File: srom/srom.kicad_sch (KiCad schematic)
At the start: 20 parts, among them J1 Conn_01x03_Female, Q1 PMBT2222A, U1 4075, U101 74LS245, U4 74LS245, U5 Pico-1 ROM

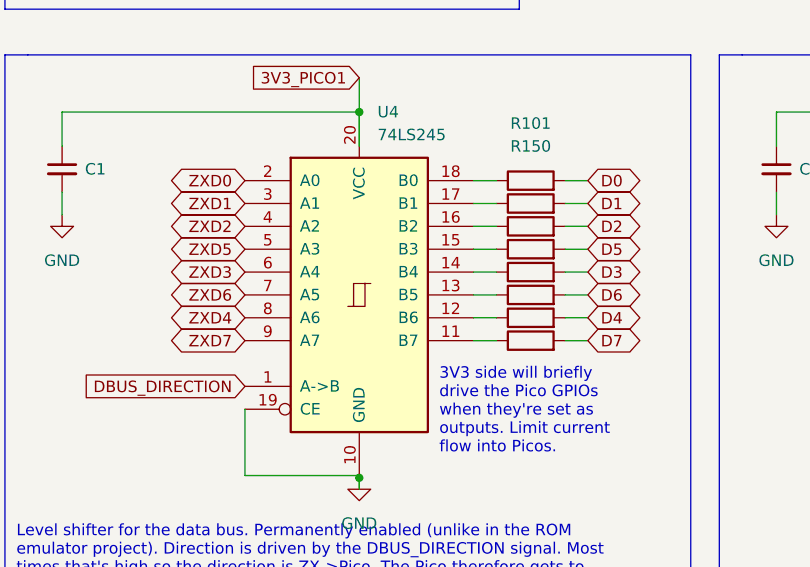
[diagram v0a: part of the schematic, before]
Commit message: first draft of layout of board 2
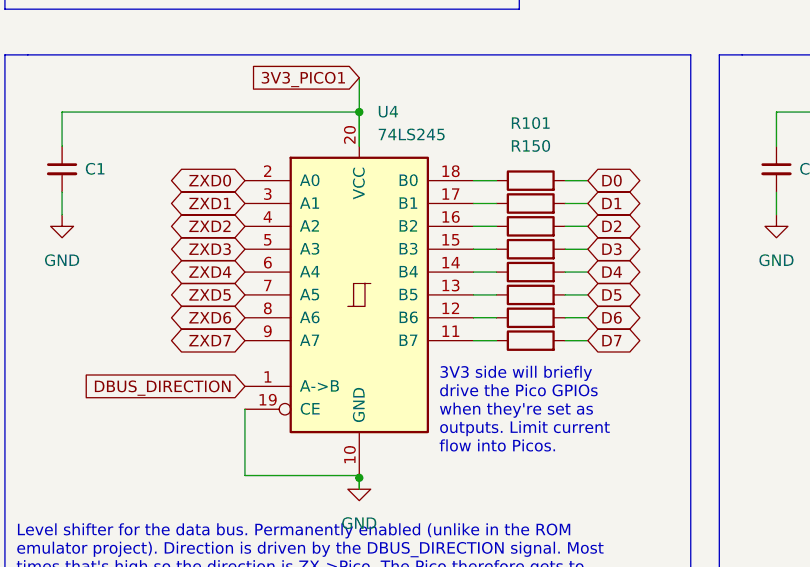
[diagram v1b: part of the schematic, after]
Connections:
- net D3: now also R104.2; no longer R105.2
- net D4: now also R105.2; no longer R107.2
- net D5: now also R106.2; no longer R104.2
- net D6: now also R107.2; no longer R106.2
- net ZXD3: now also U4.5 (A3); no longer U4.6 (A4)
- net ZXD4: now also U4.6 (A4); no longer U4.8 (A6)
- net ZXD5: now also U4.7 (A5); no longer U4.5 (A3)
- net ZXD6: now also U4.8 (A6); no longer U4.7 (A5)
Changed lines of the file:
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@@
     )
   )
-  (global_label "D4" (shape bidirectional) (at 78.74 138.43 0) (fields_autoplaced)
+  (global_label "D6" (shape bidirectional) (at 78.74 138.43 0) (fields_autoplaced)
     (effects (font (size 1.27 1.27)) (justify left))
     (property "Intersheet References" "${INTERSHEET_REFS}" (id 0) (at 83.6326 138.3506 0)
@@
     )
   )
-  (global_label "ZXD6" (shape bidirectional) (at 40.64 135.89 180) (fields_autoplaced)
+  (global_label "ZXD5" (shape bidirectional) (at 40.64 135.89 180) (fields_autoplaced)
     (effects (font (size 1.27 1.27)) (justify right))
     (property "Intersheet References" "${INTERSHEET_REFS}" (id 0) (at 33.3283 135.8106 0)
@@
     )
   )
-  (global_label "ZXD4" (shape bidirectional) (at 40.64 138.43 180) (fields_autoplaced)
+  (global_label "ZXD6" (shape bidirectional) (at 40.64 138.43 180) (fields_autoplaced)
     (effects (font (size 1.27 1.27)) (justify right))
     (property "Intersheet References" "${INTERSHEET_REFS}" (id 0) (at 33.3283 138.3506 0)
@@
     )
   )
-  (global_label "D3" (shape bidirectional) (at 78.74 133.35 0) (fields_autoplaced)
+  (global_label "D4" (shape bidirectional) (at 78.74 133.35 0) (fields_autoplaced)
     (effects (font (size 1.27 1.27)) (justify left))
     (property "Intersheet References" "${INTERSHEET_REFS}" (id 0) (at 83.6326 133.2706 0)
@@
     )
   )
-  (global_label "ZXD5" (shape bidirectional) (at 40.64 130.81 180) (fields_autoplaced)
+  (global_label "ZXD3" (shape bidirectional) (at 40.64 130.81 180) (fields_autoplaced)
     (effects (font (size 1.27 1.27)) (justify right))
     (property "Intersheet References" "${INTERSHEET_REFS}" (id 0) (at 33.3283 130.7306 0)
@@
     )
   )
-  (global_label "D6" (shape bidirectional) (at 78.74 135.89 0) (fields_autoplaced)
+  (global_label "D5" (shape bidirectional) (at 78.74 135.89 0) (fields_autoplaced)
     (effects (font (size 1.27 1.27)) (justify left))
     (property "Intersheet References" "${INTERSHEET_REFS}" (id 0) (at 83.6326 135.8106 0)
@@
     )
   )
-  (global_label "D5" (shape bidirectional) (at 78.74 130.81 0) (fields_autoplaced)
+  (global_label "D3" (shape bidirectional) (at 78.74 130.81 0) (fields_autoplaced)
     (effects (font (size 1.27 1.27)) (justify left))
     (property "Intersheet References" "${INTERSHEET_REFS}" (id 0) (at 83.6326 130.7306 0)
@@
     )
   )
-  (global_label "ZXD3" (shape bidirectional) (at 40.64 133.35 180) (fields_autoplaced)
+  (global_label "ZXD4" (shape bidirectional) (at 40.64 133.35 180) (fields_autoplaced)
     (effects (font (size 1.27 1.27)) (justify right))
     (property "Intersheet References" "${INTERSHEET_REFS}" (id 0) (at 33.3283 133.2706 0)
@@
       (reference "#PWR0201") (unit 1) (value "GND") (footprint "")
     )
+    (path "/95a6eb69-d4c1-4a7e-a8e8-144430faf0e2/49643f1b-a3e7-406d-9651-75cb8bc3c20f"
+      (reference "#PWR0202") (unit 1) (value "GND") (footprint "")
+    )
     (path "/95a6eb69-d4c1-4a7e-a8e8-144430faf0e2/b4561307-559f-491e-95d1-1c57e89e9bd0"
       (reference "#PWR0203") (unit 1) (value "GND") (footprint "")
@@
       (reference "C101") (unit 1) (value "C_Small") (footprint "Capacitor_SMD:C_1206_3216Metric")
     )
+    (path "/95a6eb69-d4c1-4a7e-a8e8-144430faf0e2/bc372065-041b-4223-9621-9581521839ff"
+      (reference "C201") (unit 1) (value "C_Small") (footprint "Capacitor_SMD:C_1206_3216Metric")
+    )
     (path "/986f0686-4dd2-4d11-a20b-857347ffd112"

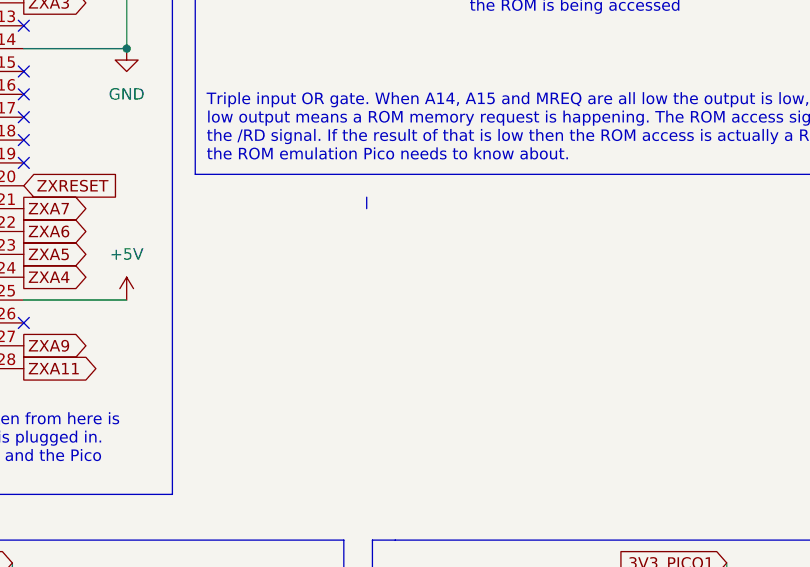
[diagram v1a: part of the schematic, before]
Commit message: more work on the layout of board 2
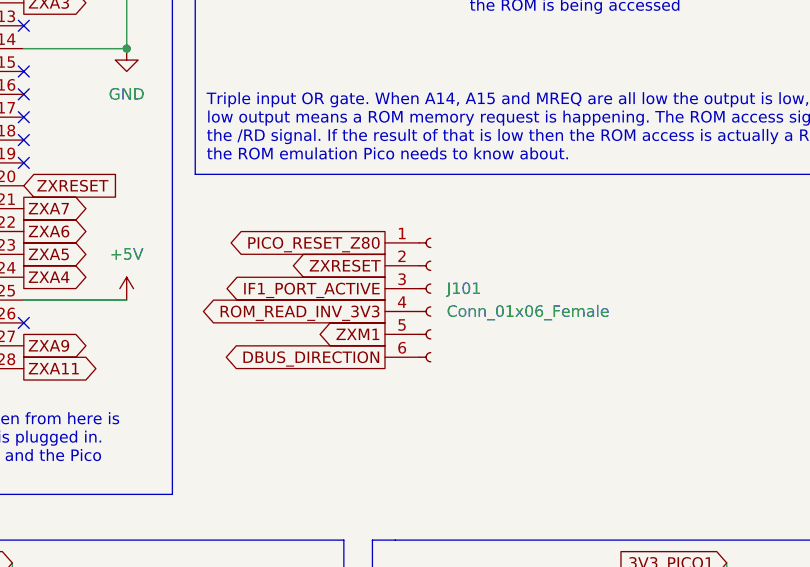
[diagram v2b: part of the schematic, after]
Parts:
- added J101: Conn_01x06_Female, Connector_PinHeader_2.54mm:PinHeader_1x06_P2.54mm_Vertical, symbol Connector:Conn_01x06_Female
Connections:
- net DBUS_DIRECTION: now also J101.6 (Pin_6)
- net IF1_PORT_ACTIVE: now also J101.3 (Pin_3)
- net PICO_RESET_Z80: now also J101.1 (Pin_1)
- net ROM_READ_INV_3V3: now also J101.4 (Pin_4)
- net ZXM1: now also J101.5 (Pin_5)
- net ZXRESET: now also J101.2 (Pin_2)
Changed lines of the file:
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@@
     (stroke (width 0) (type default) (color 0 0 0 0))
   )
-  (polyline (pts (xy 92.71 72.39) (xy 92.71 72.39))
+  (polyline (pts (xy 95.504 73.152) (xy 95.504 73.152))
     (stroke (width 0) (type default) (color 0 0 0 0))
   )
@@
   )
   (wire (pts (xy 99.695 124.46) (xy 99.695 127))
-    (stroke (width 0) (type default) (color 0 0 0 0))
-  )
-  (polyline (pts (xy 92.71 71.12) (xy 92.71 72.39))
     (stroke (width 0) (type default) (color 0 0 0 0))
   )
@@
     )
   )
+  (global_label "PICO_RESET_Z80" (shape output) (at 94.742 76.2 180) (fields_autoplaced)
+    (effects (font (size 1.27 1.27)) (justify right))
+    (property "Intersheet References" "${INTERSHEET_REFS}" (id 0) (at 76.5446 76.2794 0)
+      (effects (font (size 1.27 1.27)) (justify right) hide)
+    )
+  )
   (global_label "ZXA15" (shape output) (at 26.67 21.59 180) (fields_autoplaced)
     (effects (font (size 1.27 1.27)) (justify right))
@@
     )
   )
+  (global_label "ZXRESET" (shape output) (at 94.742 78.74 180) (fields_autoplaced)
+    (effects (font (size 1.27 1.27)) (justify right))
+    (property "Intersheet References" "${INTERSHEET_REFS}" (id 0) (at 84.1646 78.6606 0)
+      (effects (font (size 1.27 1.27)) (justify right) hide)
+    )
+  )
   (global_label "ZXD6" (shape bidirectional) (at 26.67 41.91 180) (fields_autoplaced)
     (effects (font (size 1.27 1.27)) (justify right))
@@
     )
   )
+  (global_label "ROM_READ_INV_3V3" (shape output) (at 94.742 83.82 180) (fields_autoplaced)
+    (effects (font (size 1.27 1.27)) (justify right))
+    (property "Intersheet References" "${INTERSHEET_REFS}" (id 0) (at 74.0651 83.8994 0)
+      (effects (font (size 1.27 1.27)) (justify right) hide)
+    )
+  )
   (global_label "ZXA11" (shape input) (at 242.57 67.31 0) (fields_autoplaced)
     (effects (font (size 1.27 1.27)) (justify left))
@@
     )
   )
+  (global_label "DBUS_DIRECTION" (shape output) (at 94.742 88.9 180) (fields_autoplaced)
+    (effects (font (size 1.27 1.27)) (justify right))
+    (property "Intersheet References" "${INTERSHEET_REFS}" (id 0) (at 76.4841 88.8206 0)
+      (effects (font (size 1.27 1.27)) (justify right) hide)
+    )
+  )
   (global_label "ROM_READ_INV" (shape input) (at 120.015 123.19 180) (fields_autoplaced)
     (effects (font (size 1.27 1.27)) (justify right))
@@
     )
   )
+  (global_label "ZXM1" (shape output) (at 94.742 86.36 180) (fields_autoplaced)
+    (effects (font (size 1.27 1.27)) (justify right))
+    (property "Intersheet References" "${INTERSHEET_REFS}" (id 0) (at 87.2489 86.4394 0)
+      (effects (font (size 1.27 1.27)) (justify right) hide)
+    )
+  )
   (global_label "ZXA12" (shape input) (at 242.57 64.77 0) (fields_autoplaced)
     (effects (font (size 1.27 1.27)) (justify left))
@@
     (effects (font (size 1.27 1.27)) (justify right))
     (property "Intersheet References" "${INTERSHEET_REFS}" (id 0) (at 181.1926 151.0506 0)
+      (effects (font (size 1.27 1.27)) (justify right) hide)
+    )
+  )
+  (global_label "IF1_PORT_ACTIVE" (shape output) (at 94.742 81.28 180) (fields_autoplaced)
+    (effects (font (size 1.27 1.27)) (justify right))
+    (property "Intersheet References" "${INTERSHEET_REFS}" (id 0) (at 76.4841 81.3594 0)
       (effects (font (size 1.27 1.27)) (justify right) hide)
     )
@@
     (pin "2")
   )
+  (symbol (lib_id "Connector:Conn_01x06_Female") (at 99.822 81.28 0) (unit 1)
+    (in_bom yes) (on_board yes) (fields_autoplaced)
+    (property "Reference" "J101" (id 0) (at 101.6 81.2799 0)
+      (effects (font (size 1.27 1.27)) (justify left))
+    )
+    (property "Value" "Conn_01x06_Female" (id 1) (at 101.6 83.8199 0)
+      (effects (font (size 1.27 1.27)) (justify left))
+    )
+    (property "Footprint" "Connector_PinHeader_2.54mm:PinHeader_1x06_P2.54mm_Vertical" (id 2) (at 99.822 81.28 0)
+      (effects (font (size 1.27 1.27)) hide)
+    )
+    (property "Datasheet" "~" (id 3) (at 99.822 81.28 0)
+      (effects (font (size 1.27 1.27)) hide)
+    )
+    (pin "1")
+    (pin "2")
+    (pin "3")
+    (pin "4")
+    (pin "5")
+    (pin "6")
+  )
   (symbol (lib_id "Device:R") (at 72.39 128.27 90) (unit 1)
     (in_bom yes) (on_board yes) (fields_autoplaced)
@@
       (reference "J1") (unit 1) (value "Conn_01x03_Female") (footprint "Connector_PinHeader_2.54mm:PinHeader_1x03_P2.54mm_Vertical")
     )
+    (path "/b001f89d-9f48-429a-b10f-bfc22b561bf3"
+      (reference "J101") (unit 1) (value "Conn_01x06_Female") (footprint "Connector_PinHeader_2.54mm:PinHeader_1x06_P2.54mm_Vertical")
+    )
     (path "/95a6eb69-d4c1-4a7e-a8e8-144430faf0e2/7fe63843-f758-4c7e-a4e3-75a239e41188"
       (reference "J201") (unit 1) (value "Conn_01x03_Female") (footprint "Connector_PinHeader_2.54mm:PinHeader_1x03_P2.54mm_Vertical")
     )
+    (path "/95a6eb69-d4c1-4a7e-a8e8-144430faf0e2/cd66f60d-1058-4213-bc50-c2c04efac531"
+      (reference "J202") (unit 1) (value "Conn_01x05_Female") (footprint "Connector_PinHeader_2.54mm:PinHeader_1x05_P2.54mm_Vertical")
+    )
     (path "/acda4c69-0a65-473b-ab4f-e765252d7da2/d6d0c58d-8e9e-45da-ac9c-b6edecaf4587"
